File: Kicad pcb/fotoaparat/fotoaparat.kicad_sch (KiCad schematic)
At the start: 8 parts, among them J1 USB Konektor, J3 LCD konektor, J4 Kamera, J5 Sd Karta, U1 STM32L496RETx, U2 Regulator 3.3v, U3 MCP73833-FCI/UN

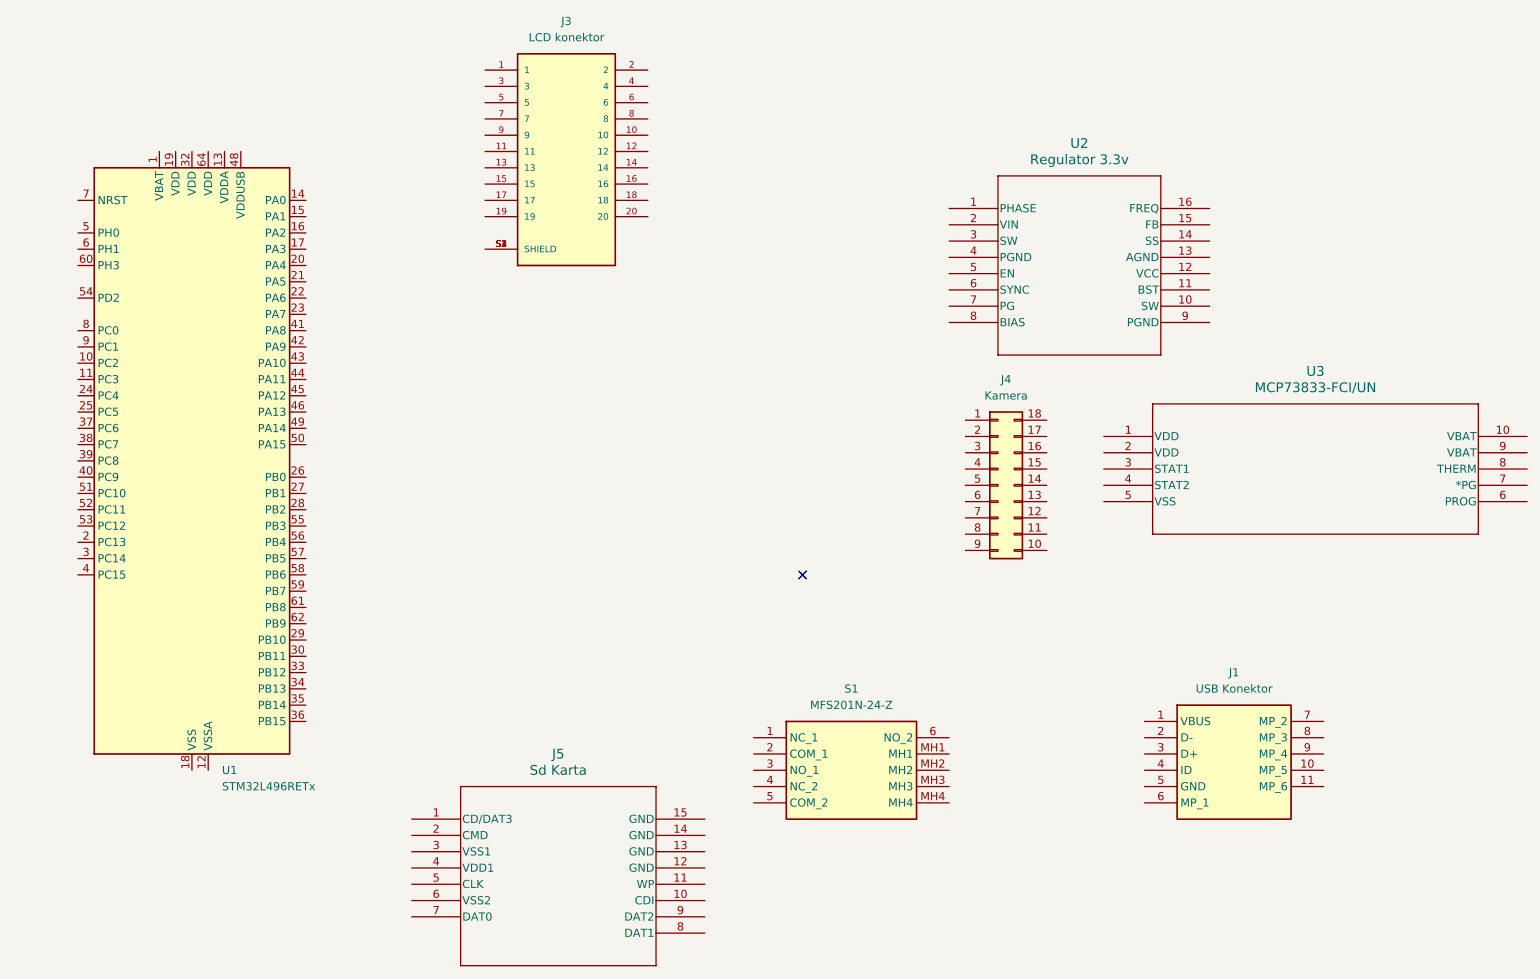
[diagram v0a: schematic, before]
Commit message: První zapojení
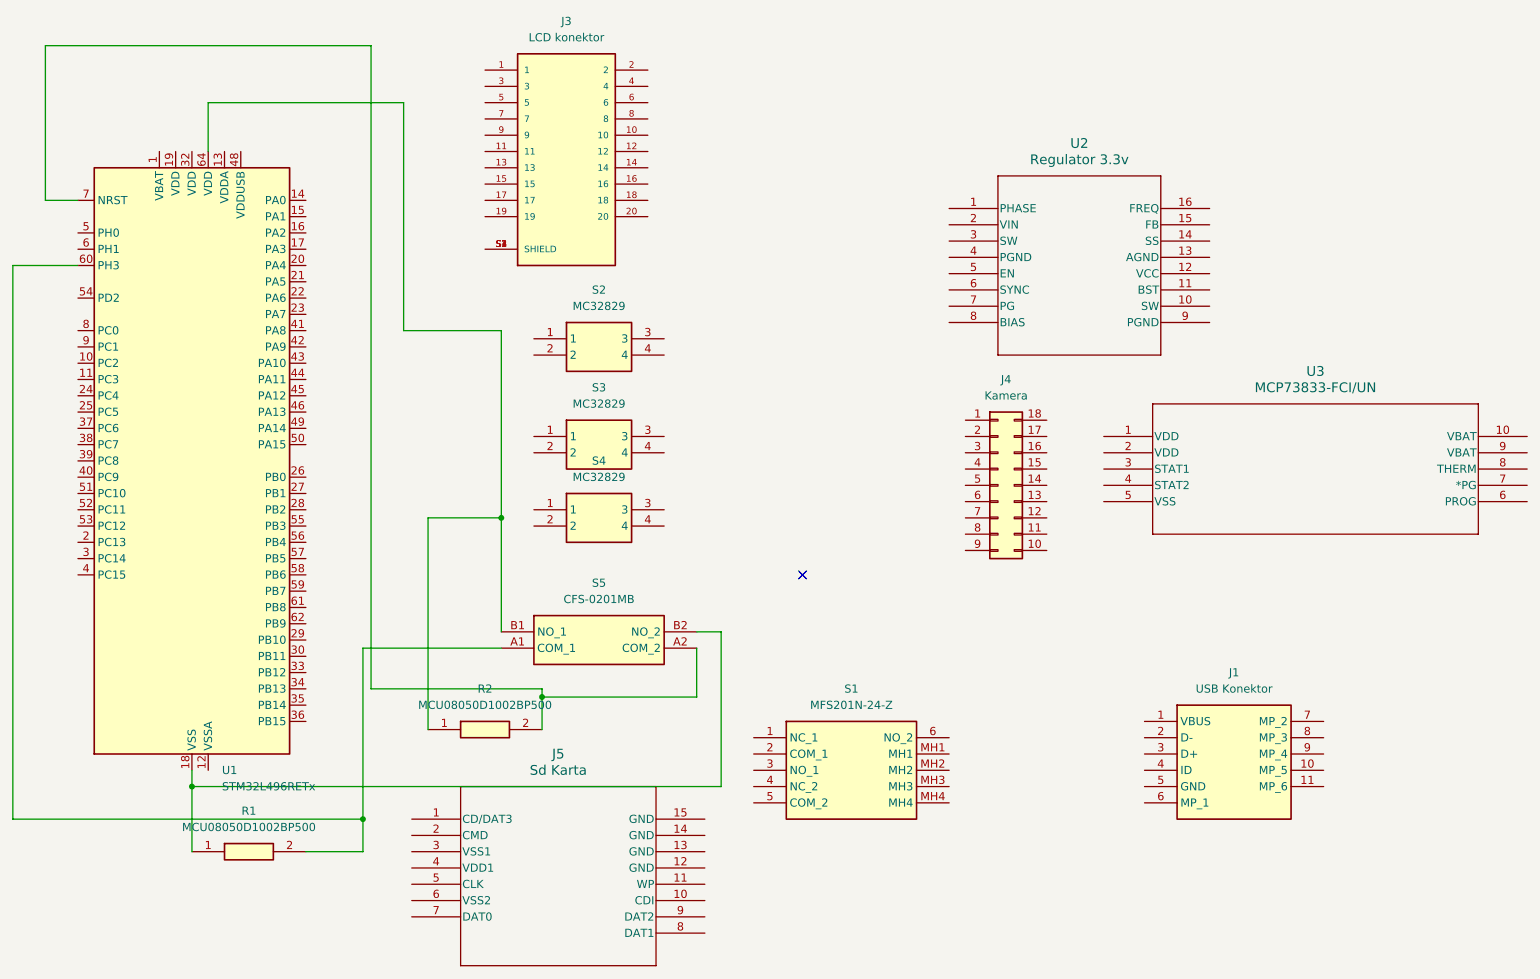
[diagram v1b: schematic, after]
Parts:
- added R1, R2: MCU08050D1002BP500, RESC2012X55N, symbol MCU08050D1002BP500:MCU08050D1002BP500
- added S2, S3, S4: MC32829, MC32829, symbol MC32829:MC32829
- added S5: CFS-0201MB, CFS0201MB, symbol CFS-0201MB:CFS-0201MB
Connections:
- net at U1.18 (VSS), U1.31 (VSS), U1.47 (VSS)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: now also R1.1, S5.B2 (NO_2)
- net at U1.60 (PH3): now also R1.2, S5.A1 (COM_1)
- net at U1.64 (VDD): now also R2.1, S5.B1 (NO_1)
- net at U1.7 (NRST): now also R2.2, S5.A2 (COM_2)
